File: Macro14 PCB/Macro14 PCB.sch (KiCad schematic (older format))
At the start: 15 parts, among them SW1 Rotary_Encoder_Switch, SW2 Rotary_Encoder_Switch, U1 Pico

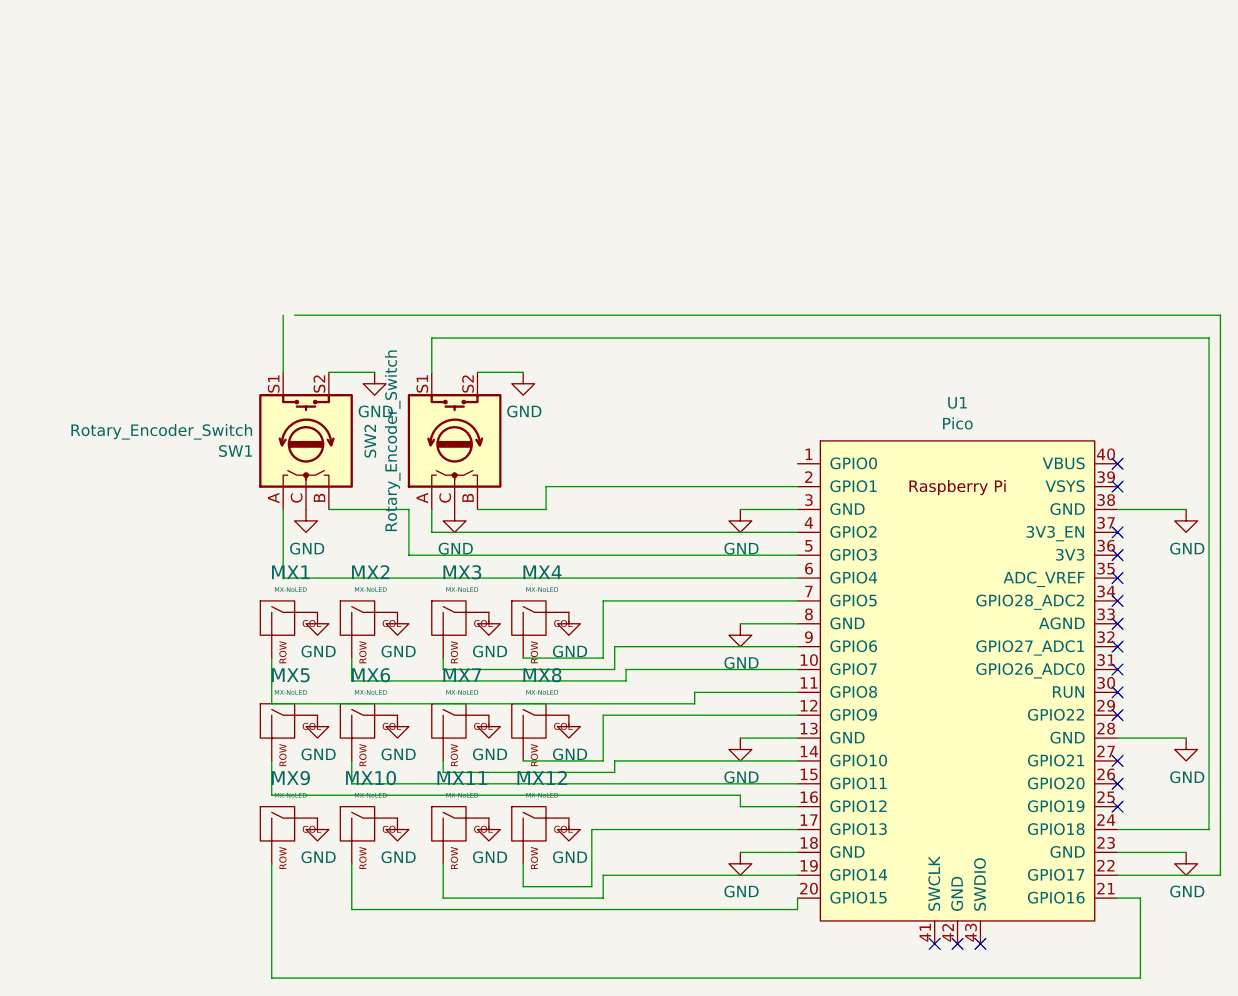
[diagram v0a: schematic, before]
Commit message: PCB completed and schematic updated
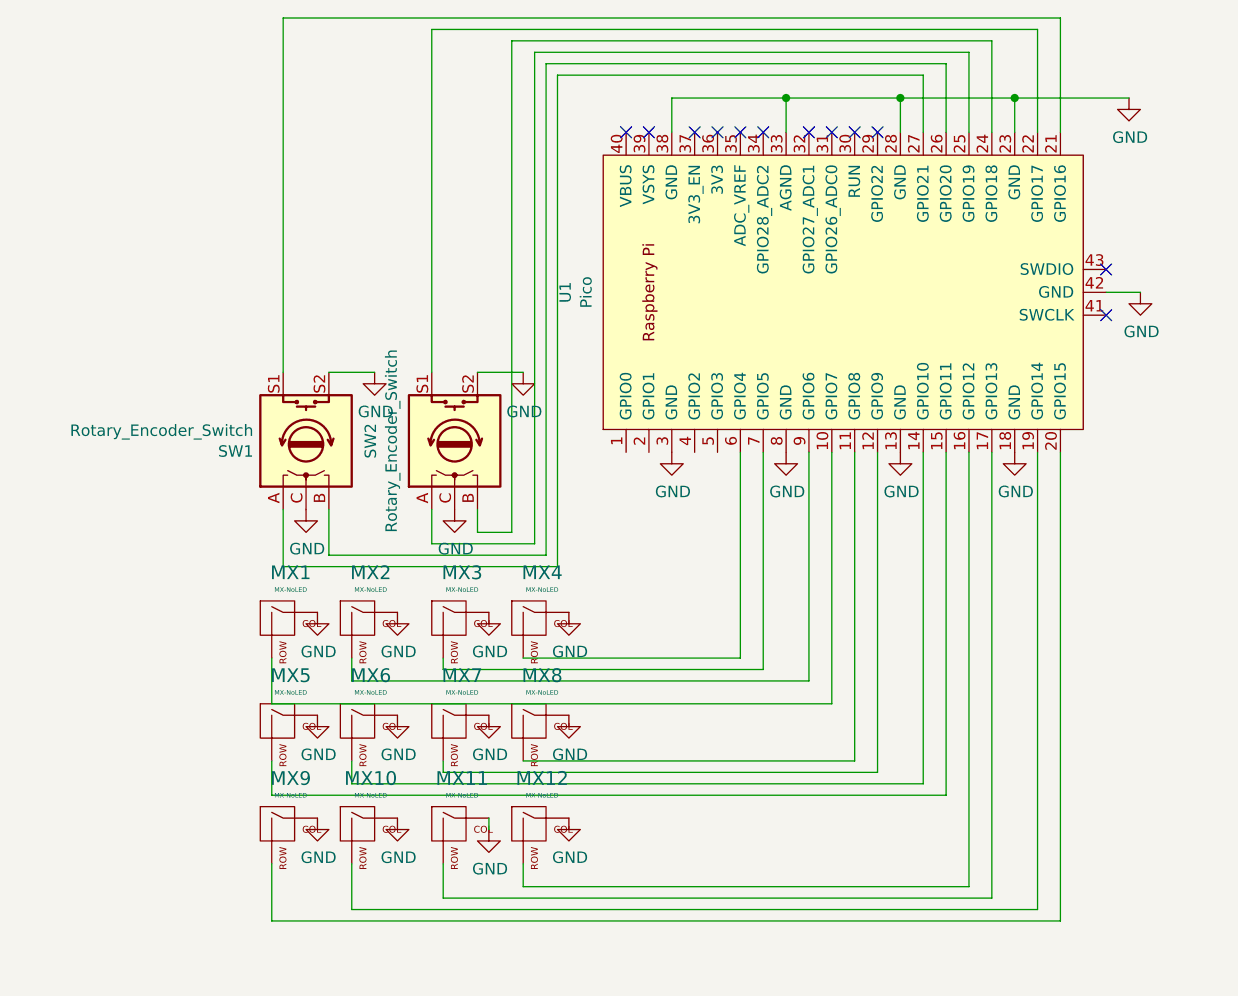
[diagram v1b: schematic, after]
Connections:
- wire segments 70 -> 72
- no-connect marks 17 -> 12
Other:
- moved on the sheet: U1
